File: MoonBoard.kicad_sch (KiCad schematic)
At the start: 23 parts, among them SW1 SW_SPST, U1 AMS1117-3.3, U10 SL2.1A, U2 STM32F446RETx, Y1 25MHz

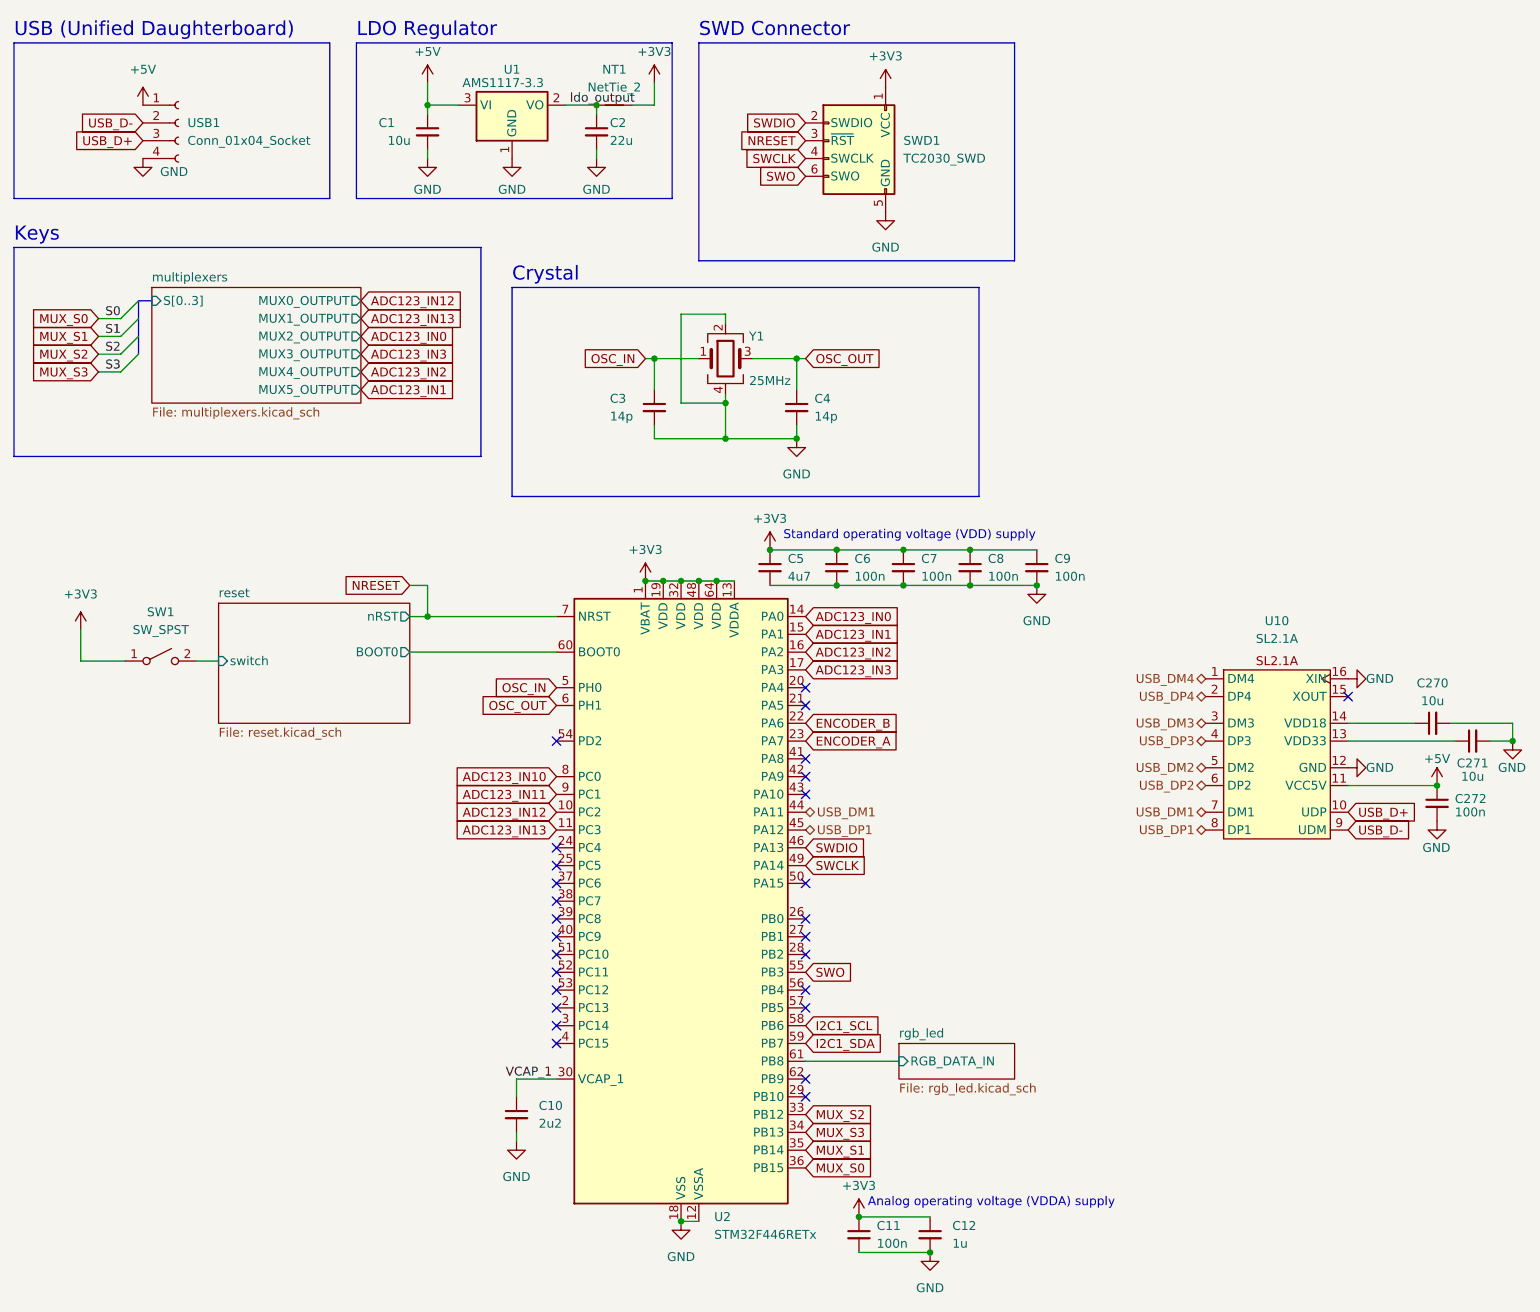
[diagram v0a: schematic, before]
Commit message: finish routing
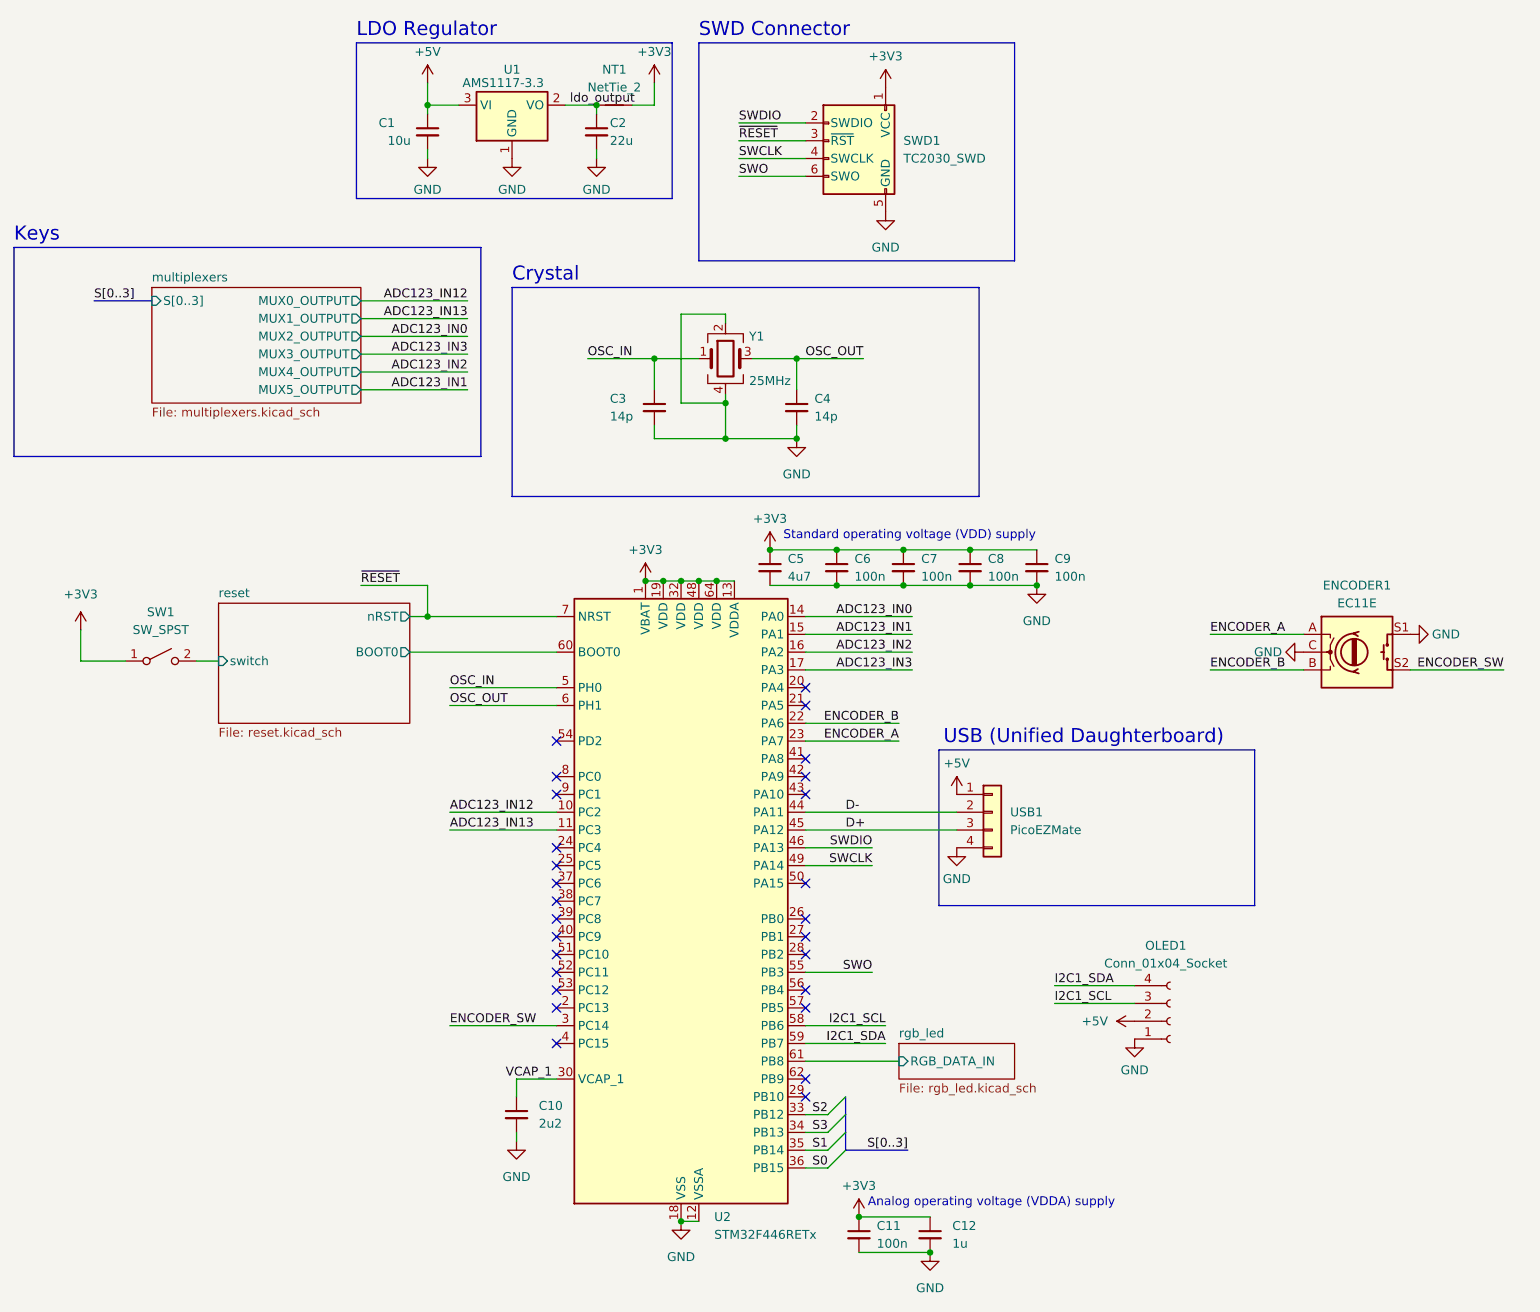
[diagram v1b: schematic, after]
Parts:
- removed C270, C271: 10u, symbol Device:C_Small
- removed C272: 100n, Capacitor_SMD:C_0402_1005Metric, symbol Device:C_Small
- removed U10: SL2.1A, MoonBoard:SSOP-16_L4.6-W2.6-P0.53-LS4.0-BL, symbol MoonBoard:SL2.1A
- removed USB1: Conn_01x04_Socket, Connector_Molex:Molex_Pico-EZmate_78171-0004_1x04-1MP_P1.20mm_Vertical, symbol Connector:Conn_01x04_Socket
- added ENCODER1: EC11E, PCM_marbastlib-various:ROT_Alps_EC11E-Switch, symbol Device:RotaryEncoder_Switch
- added OLED1: Conn_01x04_Socket, MoonBoard:OLED Module, symbol Connector:Conn_01x04_Socket
- added USB1: PicoEZMate, MoonBoard:PicoEZMate-Reinforced-Alt, symbol Connector_Generic:Conn_01x04
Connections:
- net +5V: now also OLED1.2 (Pin_2), USB1.1 (Pin_1)
- net ENCODER_A: now also ENCODER1.A
- net ENCODER_B: now also ENCODER1.B
- net GND: now also ENCODER1.C, ENCODER1.S1, OLED1.1 (Pin_1), USB1.4 (Pin_4)
- net I2C1_SCL: now also OLED1.3 (Pin_3)
- net I2C1_SDA: now also OLED1.4 (Pin_4)
- net ENCODER_SW: now reaches U2.3 (PC14)
- net ENCODER_SW: now also ENCODER1.S2
- net ADC123_IN10: no longer names the net of U2.8 (PC0)
- net ADC123_IN11: no longer names the net of U2.9 (PC1)
- net MUX_S0 renamed S0
- net MUX_S1 renamed S1
- net MUX_S2 renamed S2
- net MUX_S3 renamed S3
- net NRESET renamed ~{RESET}
- net USB_DM1 renamed D-
- net D-: now also USB1.2 (Pin_2)
- net USB_DP1 renamed D+
- net D+: now also USB1.3 (Pin_3)
